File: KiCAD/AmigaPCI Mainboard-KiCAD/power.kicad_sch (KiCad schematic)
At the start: 63 parts, among them CN600 ATX-24, J600 POWER_SWITCH, J9003 Case Fan, Q600 MMBT3904, U219 74HCT04, U222 74HCT4066, U3 74HCT08, U600 74HCT14, U601 74HCT74

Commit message: Routing June 12 2023
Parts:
- H1, H10, H2, H3, H4, H5, H6, H7, H8, H9: footprint A2900:MountingHole_Pad -> MountingHole:MountingHole_4mm_Pad_Via
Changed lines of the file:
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@@
       (effects (font (size 1.27 1.27)) (justify left) hide)
     )
-    (property "Footprint" "A2900:MountingHole_Pad" (at 289.56 146.05 0)
+    (property "Footprint" "MountingHole:MountingHole_4mm_Pad_Via" (at 289.56 146.05 0)
       (effects (font (size 1.27 1.27)) hide)
     )
@@
       (effects (font (size 1.27 1.27)) (justify left) hide)
     )
-    (property "Footprint" "A2900:MountingHole_Pad" (at 279.4 151.13 0)
+    (property "Footprint" "MountingHole:MountingHole_4mm_Pad_Via" (at 279.4 151.13 0)
       (effects (font (size 1.27 1.27)) hide)
     )
@@
       (effects (font (size 1.27 1.27)) (justify left) hide)
     )
-    (property "Footprint" "A2900:MountingHole_Pad" (at 289.56 151.13 0)
+    (property "Footprint" "MountingHole:MountingHole_4mm_Pad_Via" (at 289.56 151.13 0)
       (effects (font (size 1.27 1.27)) hide)
     )
@@
       (effects (font (size 1.27 1.27)) (justify left) hide)
     )
-    (property "Footprint" "A2900:MountingHole_Pad" (at 269.24 151.13 0)
+    (property "Footprint" "MountingHole:MountingHole_4mm_Pad_Via" (at 269.24 151.13 0)
       (effects (font (size 1.27 1.27)) hide)
     )
@@
       (effects (font (size 1.27 1.27)) (justify left) hide)
     )
-    (property "Footprint" "A2900:MountingHole_Pad" (at 279.4 146.05 0)
+    (property "Footprint" "MountingHole:MountingHole_4mm_Pad_Via" (at 279.4 146.05 0)
       (effects (font (size 1.27 1.27)) hide)
     )
@@
       (effects (font (size 1.27 1.27)) (justify left) hide)
     )
-    (property "Footprint" "A2900:MountingHole_Pad" (at 279.4 156.21 0)
+    (property "Footprint" "MountingHole:MountingHole_4mm_Pad_Via" (at 279.4 156.21 0)
       (effects (font (size 1.27 1.27)) hide)
     )
@@
       (effects (font (size 1.27 1.27)) (justify left) hide)
     )
-    (property "Footprint" "A2900:MountingHole_Pad" (at 269.24 146.05 0)
+    (property "Footprint" "MountingHole:MountingHole_4mm_Pad_Via" (at 269.24 146.05 0)
       (effects (font (size 1.27 1.27)) hide)
     )
@@
       (effects (font (size 1.27 1.27)) (justify left) hide)
     )
-    (property "Footprint" "A2900:MountingHole_Pad" (at 289.56 156.21 0)
+    (property "Footprint" "MountingHole:MountingHole_4mm_Pad_Via" (at 289.56 156.21 0)
       (effects (font (size 1.27 1.27)) hide)
     )
@@
       (effects (font (size 1.27 1.27)) (justify left) hide)
     )
-    (property "Footprint" "A2900:MountingHole_Pad" (at 289.56 160.655 0)
+    (property "Footprint" "MountingHole:MountingHole_4mm_Pad_Via" (at 289.56 160.655 0)
       (effects (font (size 1.27 1.27)) hide)
     )
@@
       (effects (font (size 1.27 1.27)) (justify left) hide)
     )
-    (property "Footprint" "A2900:MountingHole_Pad" (at 269.24 156.21 0)
-      (effects (font (size 1.27 1.27)) hide)
-    )
+    (property "Footprint" "MountingHole:MountingHole_4mm_Pad_Via" (at 269.24 156.21 0)
+      (effects (font (size 1.27 1.27)) hide)
+    )

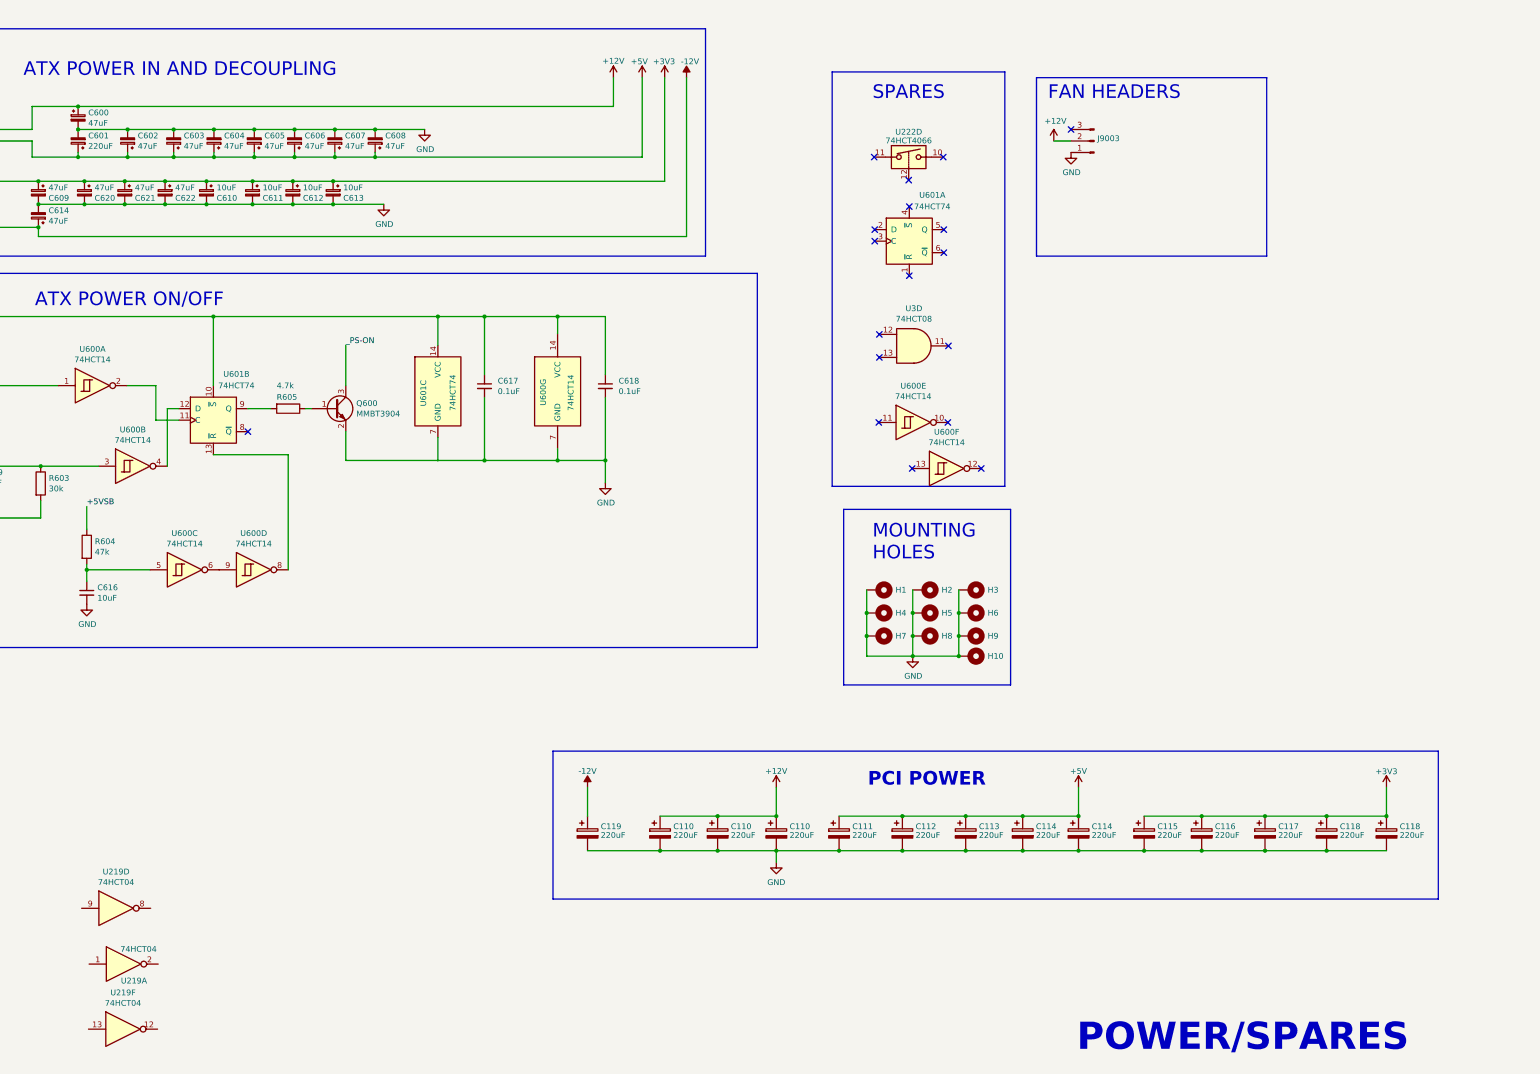
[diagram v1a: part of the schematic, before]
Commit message: Routing June 14 2023
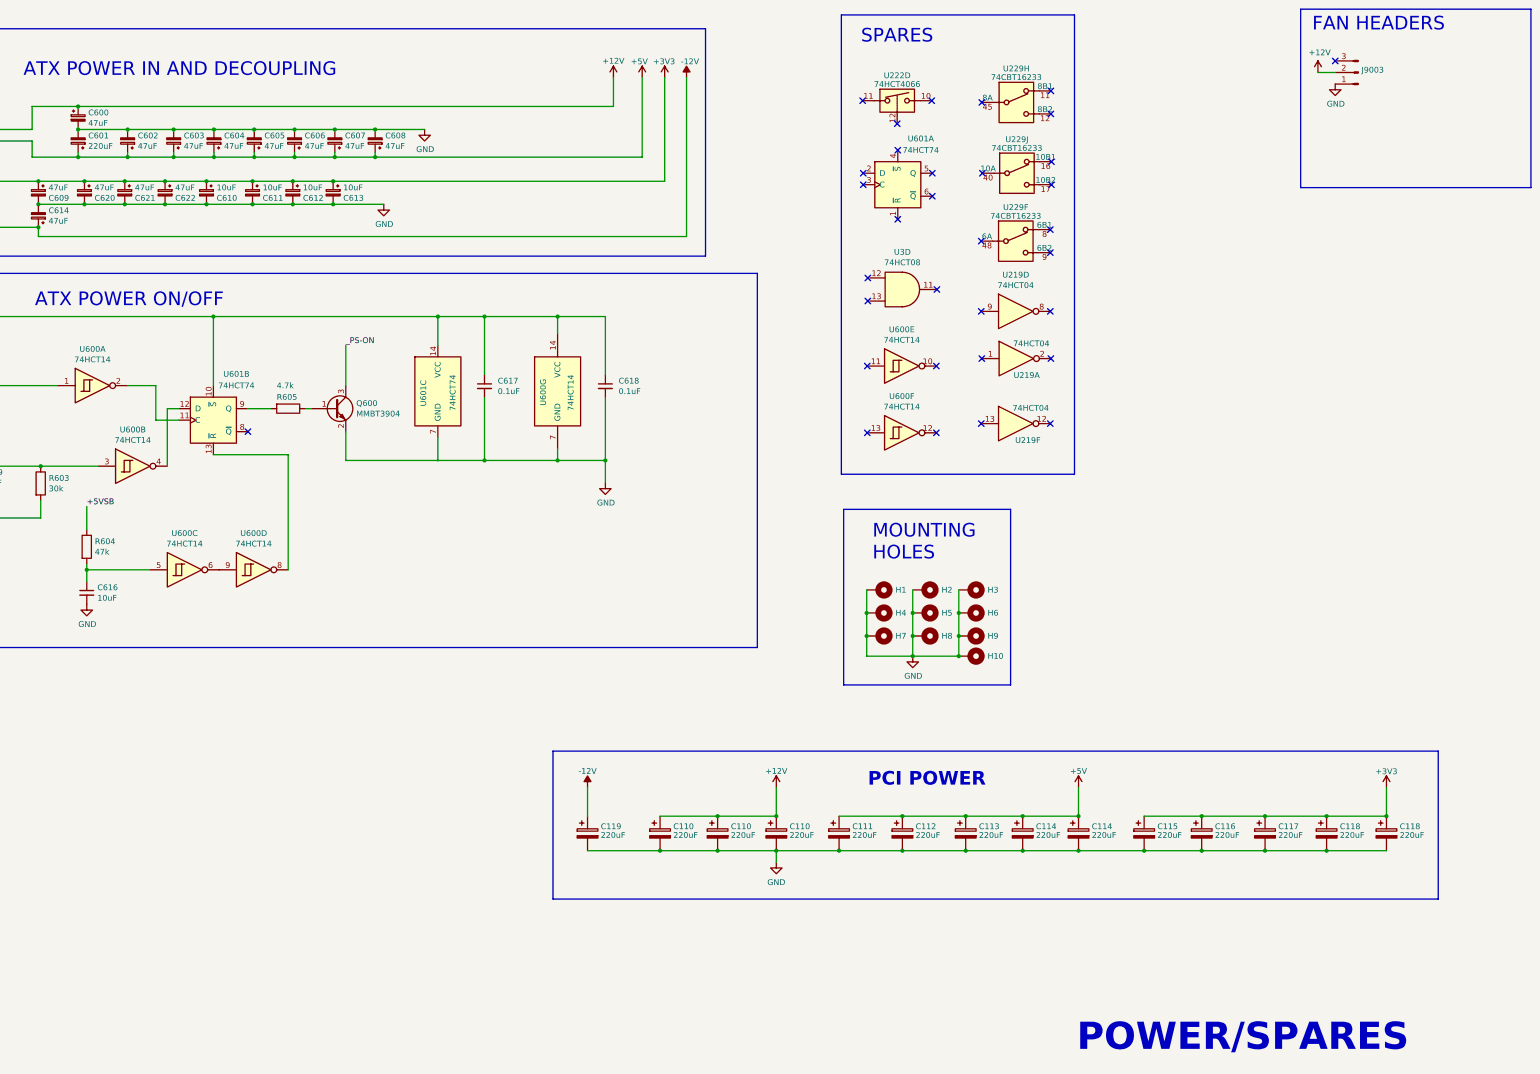
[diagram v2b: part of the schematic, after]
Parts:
- added U229: 74CBT16233, Package_SO:SSOP-56_7.5x18.5mm_P0.635mm, symbol AmigaPCI-Symbols:74CBT16233
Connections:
- no-connect marks 19 -> 34
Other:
- moved on the sheet: J9003, U219A, U219D, U219F, U222D, U3D, U600E, U600F, U601A

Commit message: Routing June 16 2023
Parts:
- U229: Part Number (none) -> SN74CBT16233DL
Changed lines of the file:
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@@
+      (effects (font (size 1.27 1.27)) hide)
+    )
+    (property "Part Number" "SN74CBT16233DL" (at 299.593 69.088 0)
       (effects (font (size 1.27 1.27)) hide)
     )
@@
       (effects (font (size 1.27 1.27)) hide)
     )
+    (property "Part Number" "SN74CBT16233DL" (at 299.72 38.481 0)
+      (effects (font (size 1.27 1.27)) hide)
+    )
     (pin "1")
     (pin "55")
@@
       (effects (font (size 1.27 1.27)) hide)
     )
+    (property "Part Number" "SN74CBT16233DL" (at 299.847 54.102 0)
+      (effects (font (size 1.27 1.27)) hide)
+    )
